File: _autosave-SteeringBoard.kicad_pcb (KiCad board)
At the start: 2 copper layers, 41.8 x 28 mm, 55 parts, among them J1 SWD, J2 Conn_01x02_Pin, J3 Conn_02x05_Counter_Clockwise, J4 Conn_01x04_Pin, SW1 Reset, U1 STM32L431CBTx, U2 ISO1044BD, U3 CDSOT23-T24CAN, U4 TPS562231DRLR, U5 RO-123.3S

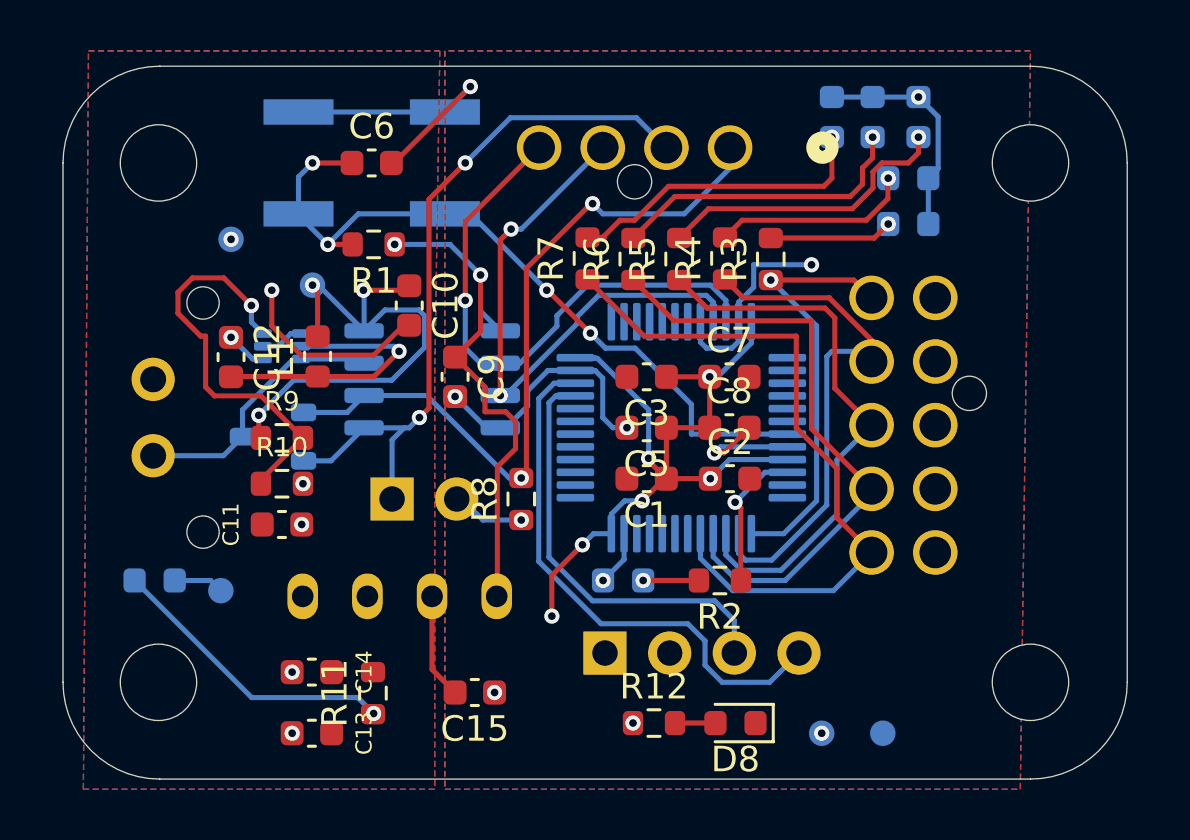
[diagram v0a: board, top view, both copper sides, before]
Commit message: finished board with ldo
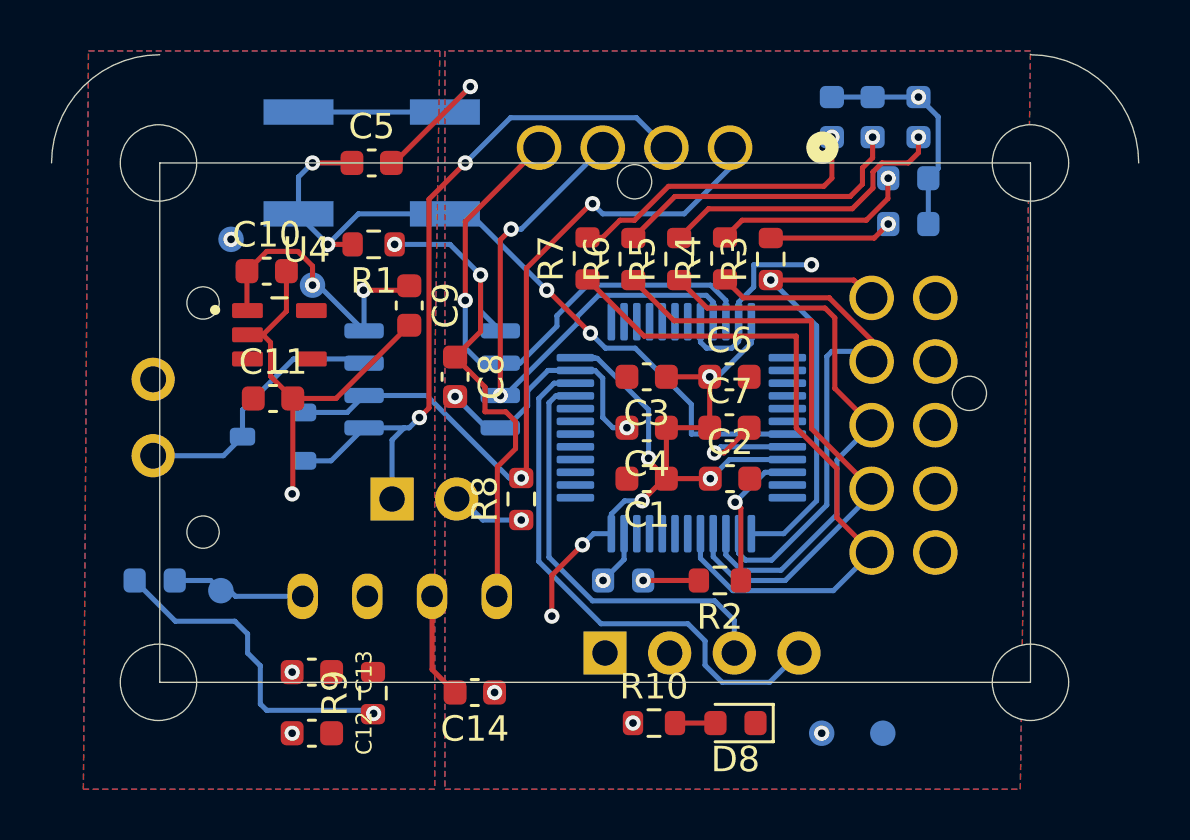
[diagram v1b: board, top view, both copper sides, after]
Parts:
- removed the C12 at (128.6, 92.6)
- removed L1: 3.3uH, Inductor_SMD:L_0603_1608Metric
- removed the R10 at (130.6, 97.6)
- removed the R9 at (130.6, 95.8)
- added C10: 1nF, Capacitor_SMD:C_0603_1608Metric, F.Cu at (130.0, 89.2)
- C11: value 10uF -> 100nF
- U4: value TPS562231DRLR -> TLV70130DBVR; footprint Package_TO_SOT_SMD:SOT-563 -> UTSVT_Power:SOT95P280X145-5N; moved to F.Cu
- moved C11 4.96 mm to (130.2, 94.2)
- moved U4 0.46 mm to (130.5, 91.8), turned to 0 degrees
- renumbered C13 to C12, C14 to C13, C15 to C14, C5 to C4, C6 to C5, C7 to C6, C8 to C7, C9 to C8, C10 to C9, R12 to R10, R11 to R9
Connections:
- C11 pad 1: /12V_Ext -> +12V
- U4 pad 1: /12V_Ext -> /3V3_Bus
- U4 pad 2: /PowerDist/SW -> GNDPWR
- U4 pad 3: GNDPWR -> +12V
- U4 pad 4: /PowerDist/BST -> unconnected-(U4-NC-Pad4)
- U4 pad 5: /12V_Ext -> unconnected-(U4-NC-Pad5)
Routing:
- net /PowerDist/FB: track 16.1 -> 0.00 mm, vias 1 -> 0
- net GNDPWR: track 19.8 -> 31.6 mm, vias 5 -> 3
- net /PowerDist/SW: track 10.9 -> 0.00 mm, vias 1 -> 0
- net /3V3_Bus: track 20.3 -> 11.2 mm, vias 3 -> 2
- net /12V_Ext: track 1.71 -> 0.00 mm
- net /PowerDist/BST: track 1.60 -> 0.00 mm, vias 1 -> 0
- net Net-(D7-A): track 11.6 -> 12.9 mm
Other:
- board size 41.8 x 28 mm -> 42.7 x 24.7 mm
